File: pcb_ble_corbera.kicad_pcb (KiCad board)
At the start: 2 copper layers, 47.6 x 24.8 mm, 13 parts, among them J2 Conn_02x04_Odd_Even, J4 Conn_ARM_JTAG_SWD_10, SW1 SW_Push, U1 BL652, U2 HDC1080

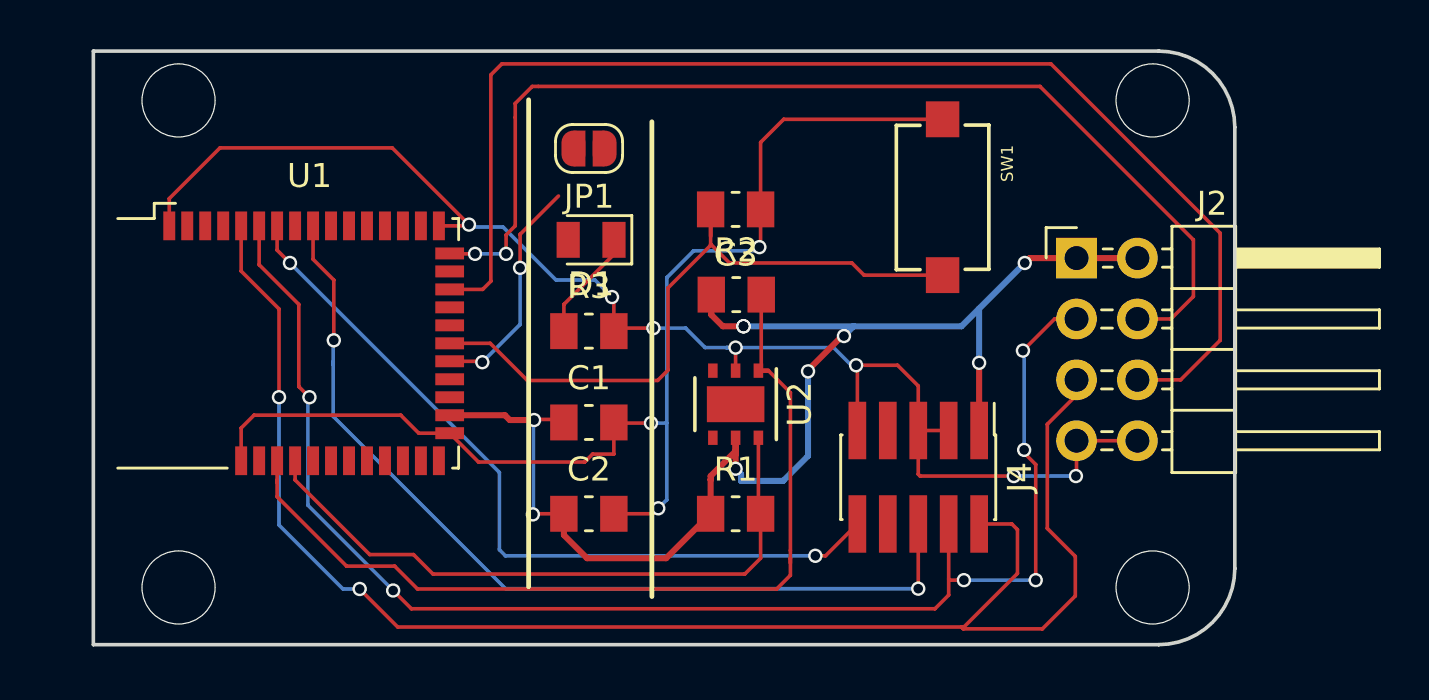
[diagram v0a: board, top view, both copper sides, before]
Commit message: updates..
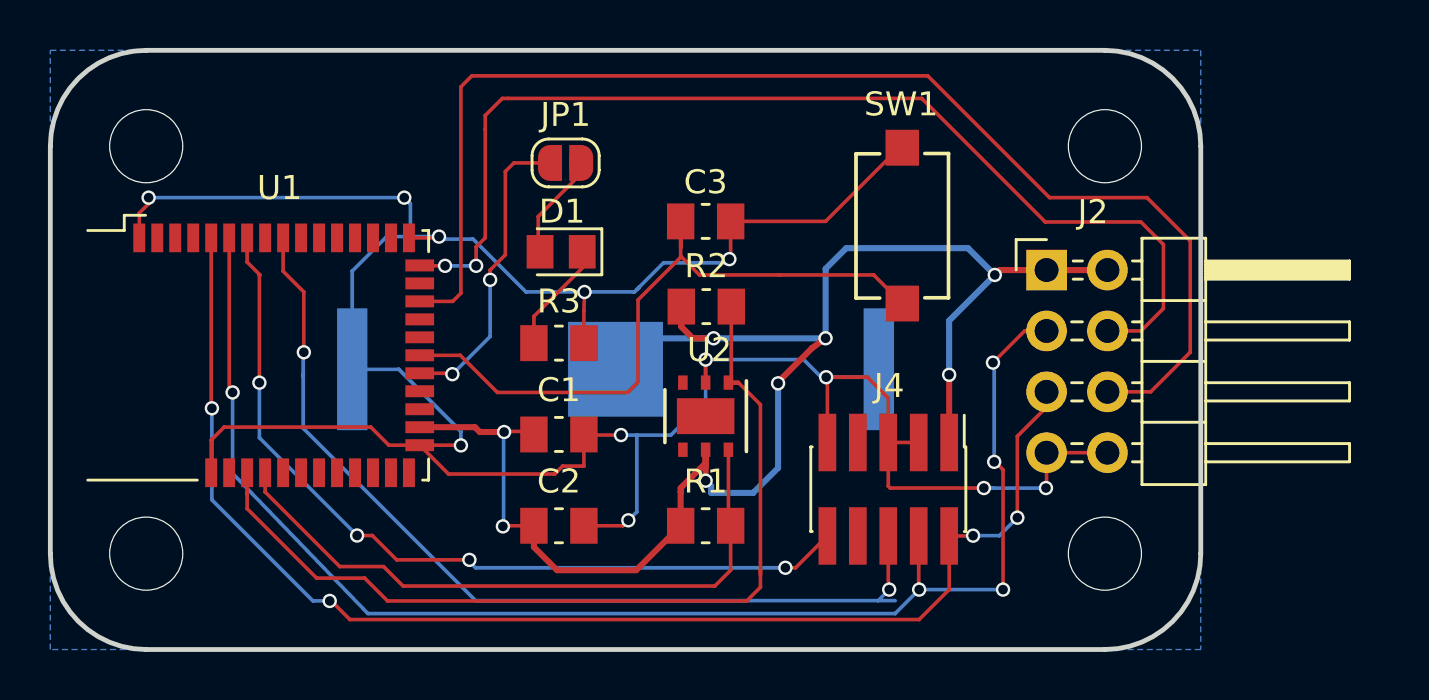
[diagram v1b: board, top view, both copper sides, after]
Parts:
- added J1: Conn_01x02, Battery_Holders:Keystone_3034_1x20mm-CoinCell, B.Cu at (151.6, 96.3)
- D1: footprint LED_SMD:LED_0805_2012Metric -> LED_SMD:LED_0805_2012Metric_Pad1.12x1.40mm_HandSolder
- JP1: footprint Jumper:SolderJumper-2_P1.3mm_Open_RoundedPad1.0x1.5mm -> TestPoint:SolderJumper-2_P1.3mm_Open_RoundedPad1.0x1.5mm
- moved SW1 2.06 mm to (163.5, 90.3)
- moved C1 1.35 mm to (149.2, 99.0)
- moved C2 1.35 mm to (149.2, 102.8)
- moved C3 1.35 mm to (155.3, 90.1)
- moved D1 1.35 mm to (149.3, 91.4)
- moved J2 1.35 mm to (169.6, 92.2)
- moved J4 1.35 mm to (163.0, 101.3)
- moved R1 1.35 mm to (155.3, 102.8)
- moved R2 1.35 mm to (155.4, 93.7)
- moved R3 1.35 mm to (149.2, 95.2)
- moved U1 1.35 mm to (137.6, 95.7)
- moved U2 1.35 mm to (155.3, 98.3)
- moved JP1 1.15 mm to (149.5, 87.7), turned to 180 degrees
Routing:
- net VCC: track 59.0 -> 70.5 mm, vias 9 -> 8
- net GND: track 109.8 -> 120.6 mm, vias 10 -> 12
- net SWDIO-TMS: track 66.3 -> 56.2 mm, vias 2 -> 4
- net Net-(D1-Pad2): track 0.00 -> 4.45 mm
- net LED_0: track 9.63 -> 12.8 mm
- net RESET: track 32.9 -> 35.1 mm, vias 2 -> 4
- net SWDCLK: track 62.0 -> 61.5 mm, vias 6 -> 5
- added copper zone on B.Cu, net GND
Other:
- board size 47.6 x 24.8 mm -> 48 x 25 mm
